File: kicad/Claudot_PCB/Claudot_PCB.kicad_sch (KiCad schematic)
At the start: 52 parts, among them J1 Conn_01x04, SW1 SW_Push, SW10 SW_Push, SW11 SW_Push, SW12 RotaryEncoder, SW2 SW_Push, SW3 SW_Push, SW4 SW_Push, SW5 SW_Push, SW6 SW_Push, SW7 SW_Push, SW8 SW_Push, SW9 SW_Push, U1 RP2040, U2 W25Q16JVUXIQ, U3 AP2112K-3.3, Y1 12MHz

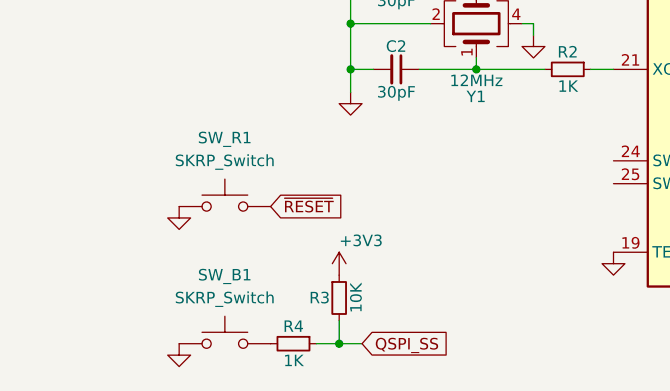
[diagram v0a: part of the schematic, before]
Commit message: Update schematic and pcb
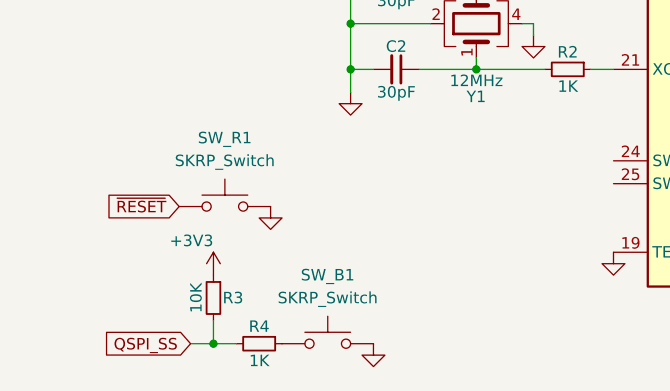
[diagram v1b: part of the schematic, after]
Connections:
- net GND: now also SW_B1.3, SW_B1.4, SW_R1.3, SW_R1.4; no longer SW_B1.1, SW_R1.1
- net QSPI_SS: now also R4.2; no longer R4.1
- net ~{RESET}: now also SW_R1.1, SW_R1.2; no longer SW_R1.3
- new net: R4.1, SW_B1.1, SW_B1.2
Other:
- moved on the sheet: R3, R4, SW_B1
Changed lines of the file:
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@@
 	)
 	(junction
-		(at 48.26 189.23)
+		(at 34.29 189.23)
 		(diameter 0)
 		(color 0 0 0 0)
@@
 	(wire
 		(pts
-			(xy 45.72 189.23) (xy 48.26 189.23)
+			(xy 36.83 189.23) (xy 34.29 189.23)
 		)
 		(stroke
@@
 	(wire
 		(pts
-			(xy 48.26 189.23) (xy 50.8 189.23)
+			(xy 34.29 189.23) (xy 31.75 189.23)
 		)
 		(stroke
@@
 	(wire
 		(pts
-			(xy 48.26 186.69) (xy 48.26 189.23)
+			(xy 34.29 186.69) (xy 34.29 189.23)
 		)
 		(stroke
@@
 	(global_label "~{RESET}"
 		(shape input)
-		(at 40.64 173.99 0)
+		(at 30.48 173.99 180)
 		(fields_autoplaced yes)
 		(effects
@@
 				(size 1.27 1.27)
 			)
-			(justify left)
+			(justify right)
 		)
 		(property "Intersheetrefs" "${INTERSHEET_REFS}"
-			(at 49.3703 173.99 0)
+			(at 21.7497 173.99 0)
 			(effects
 				(font
 					(size 1.27 1.27)
 				)
-				(justify left)
+				(justify right)
 				(hide yes)
 			)
@@
 	(global_label "QSPI_SS"
 		(shape input)
-		(at 50.8 189.23 0)
+		(at 31.75 189.23 180)
 		(fields_autoplaced yes)
 		(effects
@@
 				(size 1.27 1.27)
 			)
-			(justify left)
+			(justify right)
 		)
 		(property "Intersheetrefs" "${INTERSHEET_REFS}"
-			(at 61.5866 189.23 0)
+			(at 20.9634 189.23 0)
 			(effects
 				(font
 					(size 1.27 1.27)
 				)
-				(justify left)
+				(justify right)
 				(hide yes)
 			)
@@
 	(symbol
 		(lib_id "power:+3V3")
-		(at 48.26 181.61 0)
+		(at 34.29 181.61 0)
+		(mirror y)
 		(unit 1)
 		(exclude_from_sim no)
@@
 		(dnp no)
 		(property "Reference" "#PWR024"
-			(at 48.26 185.42 0)
+			(at 34.29 185.42 0)
 			(effects
 				(font
@@
 		)
 		(property "Value" "+3V3"
-			(at 48.26 177.8 0)
+			(at 34.29 177.8 0)
 			(effects
 				(font
@@
 		)
 		(property "Footprint" ""
-			(at 48.26 181.61 0)
+			(at 34.29 181.61 0)
 			(effects
 				(font
@@
 		)
 		(property "Datasheet" ""
-			(at 48.26 181.61 0)
+			(at 34.29 181.61 0)
 			(effects
 				(font
@@
 		)
 		(property "Description" ""
-			(at 48.26 181.61 0)
+			(at 34.29 181.61 0)
 			(effects
 				(font
@@
 	(symbol
 		(lib_id "power:GND")
-		(at 30.48 189.23 0)
+		(at 52.07 189.23 0)
+		(mirror y)
 		(unit 1)
 		(exclude_from_sim no)
@@
 		(fields_autoplaced yes)
 		(property "Reference" "#PWR027"
-			(at 30.48 195.58 0)
+			(at 52.07 195.58 0)
 			(effects
 				(font
@@
 		)
 		(property "Value" "GND"
-			(at 30.48 194.31 0)
+			(at 52.07 194.31 0)
 			(effects
 				(font
@@
 		)
 		(property "Footprint" ""
-			(at 30.48 189.23 0)
+			(at 52.07 189.23 0)
 			(effects
 				(font
@@
 		)
 		(property "Datasheet" ""
-			(at 30.48 189.23 0)
+			(at 52.07 189.23 0)
 			(effects
 				(font
@@
 		)
 		(property "Description" ""
-			(at 30.48 189.23 0)
+			(at 52.07 189.23 0)
 			(effects
 				(font
@@
 		(on_board yes)
 		(dnp no)
-		(fields_autoplaced yes)
 		(property "Reference" "SW_R1"
 			(at 35.56 166.37 0)
@@
 		(pin "3"
 		)
+		(pin "2"
+		)
+		(pin "4"
+		)
 		(instances
 			(project ""
@@
 	(symbol
 		(lib_id "Device:R_Small")
-		(at 48.26 184.15 0)
+		(at 34.29 184.15 0)
+		(mirror y)
 		(unit 1)
 		(exclude_from_sim no)
@@
 		(dnp no)
 		(property "Reference" "R3"
-			(at 47.244 184.15 0)
+			(at 35.306 184.15 0)
 			(effects
 				(font
@@
 		)
 		(property "Value" "10K"
-			(at 50.165 184.15 90)
+			(at 32.385 184.15 90)
 			(effects
 				(font
@@
 		)
 		(property "Footprint" "Resistor_SMD:R_0402_1005Metric"
-			(at 48.26 184.15 0)
+			(at 34.29 184.15 0)
 			(effects
 				(font
@@
 		)
 		(property "Datasheet" "~"
-			(at 48.26 184.15 0)
+			(at 34.29 184.15 0)
 			(effects
 				(font
@@
 		)
 		(property "Description" ""
-			(at 48.26 184.15 0)
+			(at 34.29 184.15 0)
 			(effects
 				(font
@@
 		)
 		(property "LCSC" "C25744"
-			(at 48.26 184.15 0)
+			(at 34.29 184.15 0)
 			(effects
 				(font
@@
 	(symbol
 		(lib_id "power:GND")
-		(at 30.48 173.99 0)
+		(at 40.64 173.99 0)
+		(mirror y)
 		(unit 1)
 		(exclude_from_sim no)
@@
 		(fields_autoplaced yes)
 		(property "Reference" "#PWR026"
-			(at 30.48 180.34 0)
+			(at 40.64 180.34 0)
 			(effects
 				(font
@@
 		)
 		(property "Value" "GND"
-			(at 30.48 179.07 0)
+			(at 40.64 179.07 0)
 			(effects
 				(font
@@
 		)
 		(property "Footprint" ""
-			(at 30.48 173.99 0)
+			(at 40.64 173.99 0)
 			(effects
 				(font
@@
 		)
 		(property "Datasheet" ""
-			(at 30.48 173.99 0)
+			(at 40.64 173.99 0)
 			(effects
 				(font
@@
 		)
 		(property "Description" ""
-			(at 30.48 173.99 0)
+			(at 40.64 173.99 0)
 			(effects
 				(font
@@
 	(symbol
 		(lib_id "Device:R_Small")
-		(at 43.18 189.23 270)
+		(at 39.37 189.23 270)
 		(unit 1)
 		(exclude_from_sim no)
@@
 		(dnp no)
 		(property "Reference" "R4"
-			(at 43.18 187.325 90)
+			(at 39.37 187.325 90)
 			(effects
 				(font
@@
 		)
 		(property "Value" "1K"
-			(at 43.18 191.135 90)
+			(at 39.37 191.135 90)
 			(effects
 				(font
@@
 		)
 		(property "Footprint" "Resistor_SMD:R_0402_1005Metric"
-			(at 43.18 189.23 0)
+			(at 39.37 189.23 0)
 			(effects
 				(font
@@
 		)
 		(property "Datasheet" "~"
-			(at 43.18 189.23 0)
+			(at 39.37 189.23 0)
 			(effects
 				(font
@@
 		)
 		(property "Description" ""
-			(at 43.18 189.23 0)
+			(at 39.37 189.23 0)
 			(effects
 				(font
@@
 		)
 		(property "LCSC" "C11702"
-			(at 43.18 189.23 0)
+			(at 39.37 189.23 0)
 			(effects
 				(font
@@
 	(symbol
 		(lib_id "Library:SKRP_Switch")
-		(at 35.56 189.23 0)
+		(at 46.99 189.23 0)
 		(unit 1)
 		(exclude_from_sim no)
@@
 		(on_board yes)
 		(dnp no)
-		(fields_autoplaced yes)
 		(property "Reference" "SW_B1"
-			(at 35.56 181.61 0)
+			(at 46.99 181.61 0)
 			(effects
 				(font
@@
 		)
 		(property "Value" "SKRP_Switch"
-			(at 35.56 184.15 0)
+			(at 46.99 184.15 0)
 			(effects
 				(font
@@
 		)
 		(property "Footprint" "Library:SKRP_Switch"
-			(at 35.56 184.15 0)
+			(at 46.99 184.15 0)
 			(effects
 				(font
@@
 		)
 		(property "Datasheet" ""
-			(at 35.56 184.15 0)
+			(at 46.99 184.15 0)
 			(effects
 				(font
@@
 		)
 		(property "Description" ""
-			(at 35.56 189.23 0)
+			(at 46.99 189.23 0)
 			(effects
 				(font
@@
 		(pin "3"
 		)
+		(pin "2"
+		)
+		(pin "4"
+		)
 		(instances

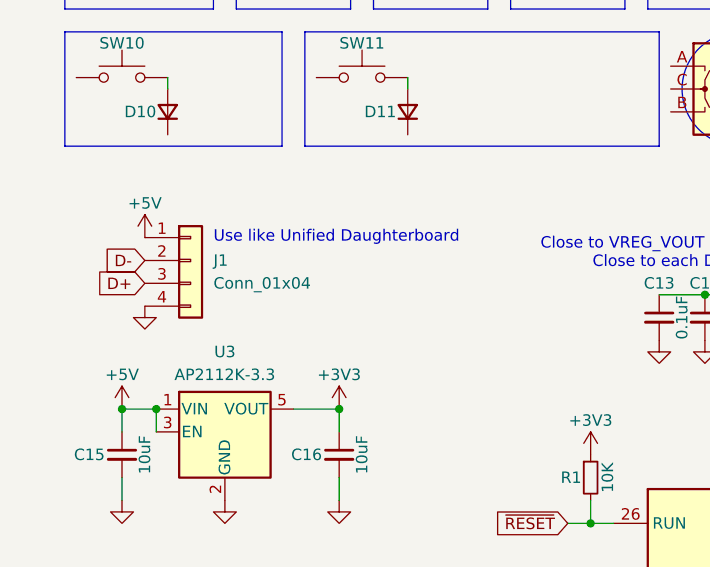
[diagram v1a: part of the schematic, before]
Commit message: Update schematic and pcb
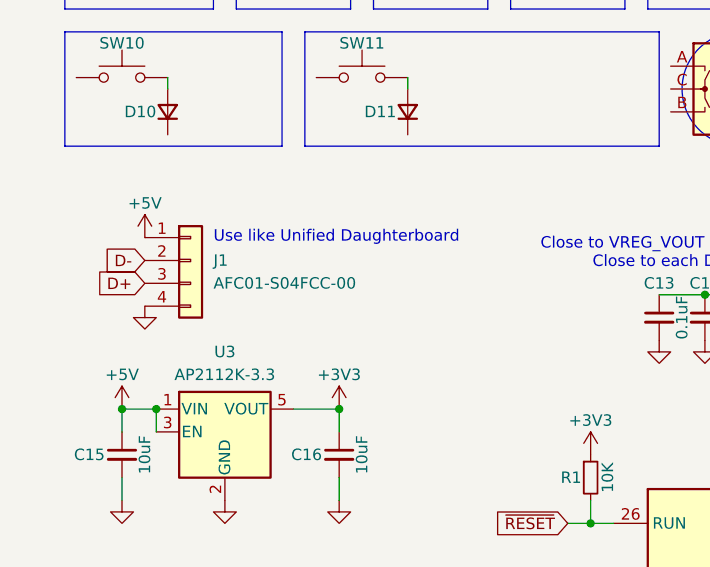
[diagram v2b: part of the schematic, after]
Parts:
- J1: value Conn_01x04 -> AFC01-S04FCC-00
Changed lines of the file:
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@@
 			)
 		)
-		(property "Value" "Conn_01x04"
+		(property "Value" "AFC01-S04FCC-00"
 			(at 34.29 76.1999 0)
 			(effects
